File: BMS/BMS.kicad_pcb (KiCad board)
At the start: 2 copper layers, 15 x 15 mm, 17 parts, among them J1 Conn_01x02_Pin, J2 Conn_01x02_Pin, J3 Conn_01x02_Pin, Q1 A03401A, U1 MCP73831-2-OT, U2 XC6206PxxxMR

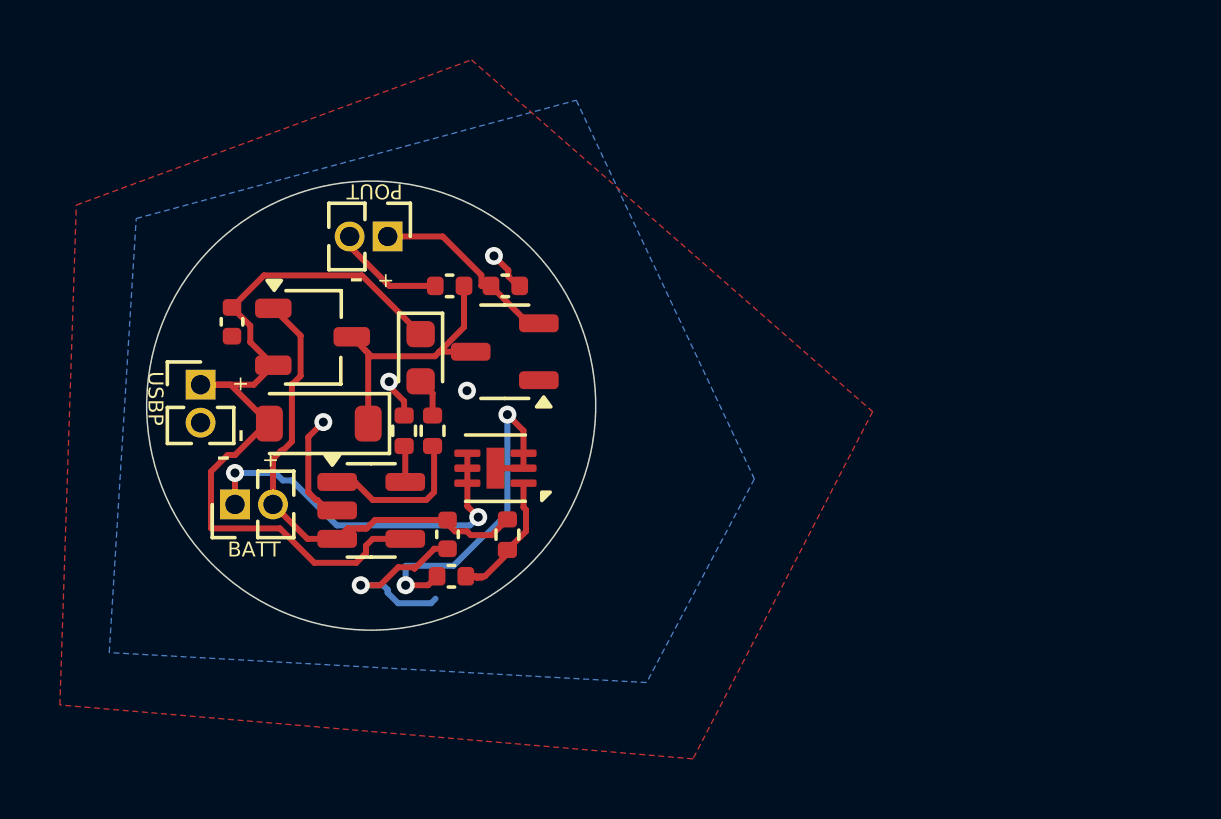
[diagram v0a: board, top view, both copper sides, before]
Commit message: BMS Rev 2
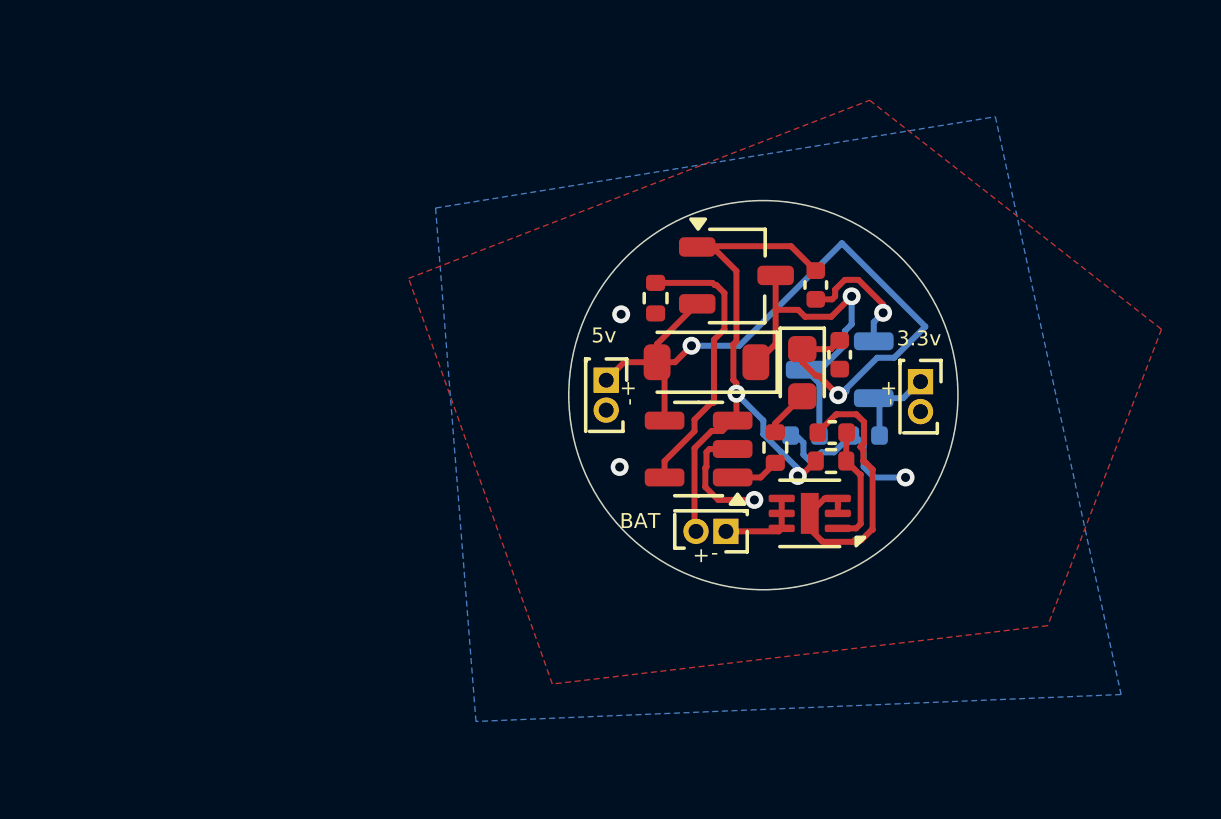
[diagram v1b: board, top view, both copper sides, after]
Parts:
- C2, C3, U2: moved to B.Cu
- J1, J2, J3: footprint Connector_PinHeader_1.27mm:PinHeader_1x02_P1.27mm_Vertical -> Connector_PinHeader_1.00mm:PinHeader_2x01_P1.00mm_Vertical
- moved C1 20.3 mm to (40.5, 17.9)
- moved J3 18.4 mm to (43.2, 18.9)
- moved J2 16.4 mm to (36.8, 23.9), turned to 180 degrees
- moved C4 14.9 mm to (39.8, 15.6)
- moved Q1 14.3 mm to (37.1, 15.3)
- moved C5 13.6 mm to (40.3, 20.6)
- moved J1 13.6 mm to (32.8, 18.8), turned to -90 degrees
- moved D1 13.1 mm to (36.1, 18.2)
- moved C3 13.0 mm to (41.4, 20.6), turned to 180 degrees
- moved C2 12.9 mm to (39.4, 20.6)
- moved D2 12.8 mm to (39.3, 18.6)
- moved R2 11.5 mm to (38.4, 21.1)
- moved U2 11.2 mm to (40.5, 18.4)
- moved U1 11.1 mm to (35.8, 21.1), turned to 180 degrees
- moved R3 11.1 mm to (40.3, 21.5), turned to 0 degrees
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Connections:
- net Net-(D1-K) renamed Vdrive
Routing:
- net Net-(J2-Pin_1): track 12.4 -> 2.90 mm, vias 2 -> 0
- net Net-(U1-PROG): track 1.22 -> 9.48 mm
- net Net-(U1-STAT): track 5.16 -> 1.63 mm
- net +3V3: track 6.46 -> 3.12 mm
- net VBAT: track 16.9 -> 19.9 mm, vias 0 -> 2
- net Vdrive: track 9.34 -> 11.9 mm, vias 0 -> 1
- net GND: track 16.6 -> 14.2 mm
- net VBUS: track 27.6 -> 25.7 mm, vias 0 -> 2
- net Net-(U3-EPAD): track 12.2 -> 10.4 mm, vias 2 -> 0
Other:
- board size 15 x 15 mm -> 13 x 13 mm
- board text added: "3.3v"
- board text added: "5v"
- board text added: "BAT"
- board text added: "MaxV: 5v"
- board text added: "Nixie Pendant BMS"
- board text added: "OutV: 3.3v"
- board text added: "Rev 2"
- board text removed: "BATT"
- board text removed: "POUT"
- board text removed: "USBP"

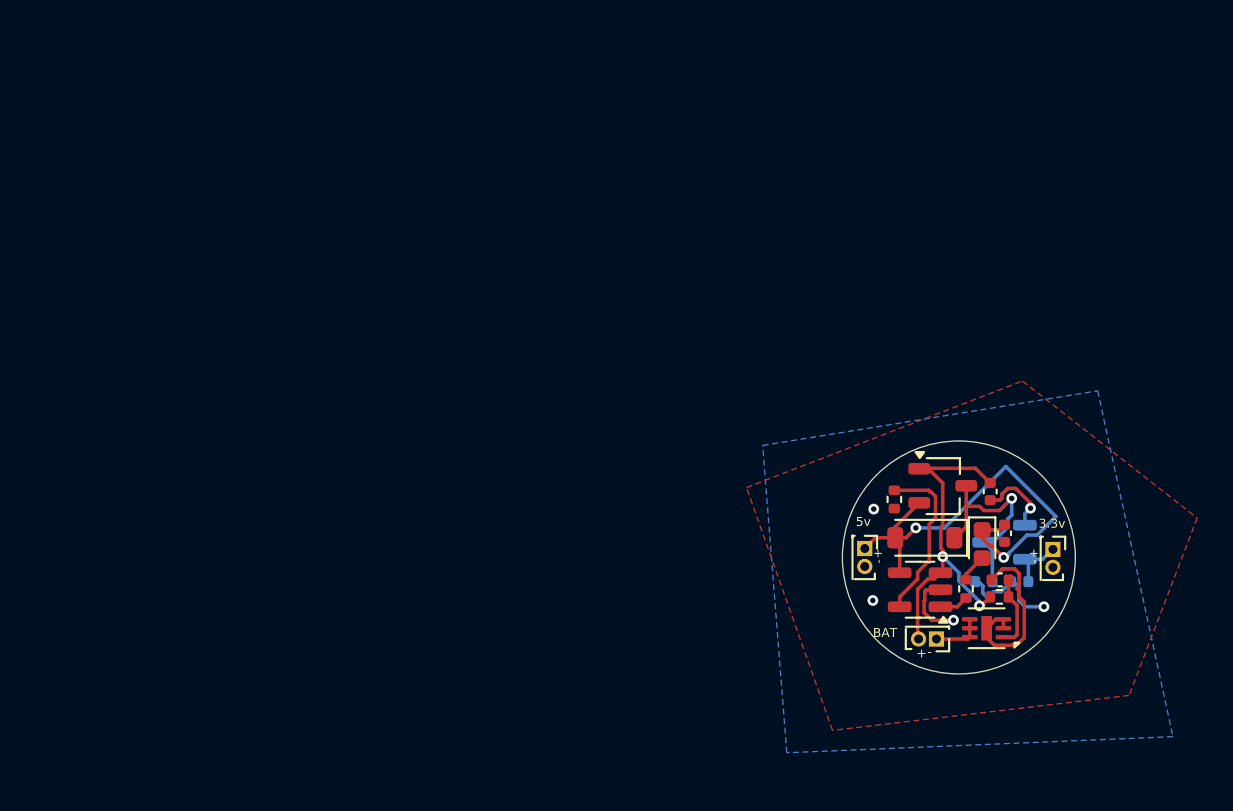
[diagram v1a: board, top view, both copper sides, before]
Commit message: Some BMS changes?, Socket PCB
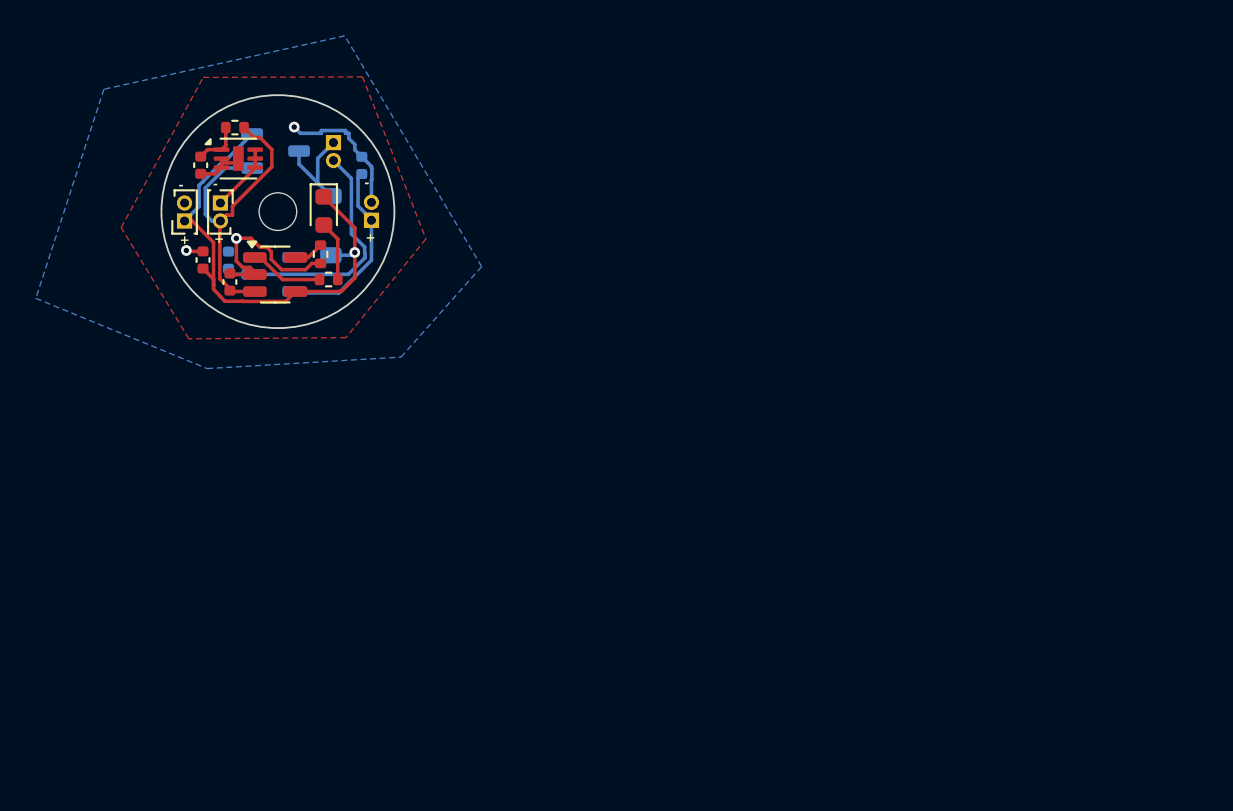
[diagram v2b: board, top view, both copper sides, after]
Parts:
- added H1: MountingHole, PendantLib:MountingHole_1.5mm, F.Cu at (0.00, 0.00)
- added SW1: SW_DPST_x2, Connector_PinHeader_1.00mm:PinHeader_2x01_P1.00mm_Vertical, B.Cu at (3.10, -3.85)
- D1, J3, Q1: moved to B.Cu
- moved C5 50.3 mm to (-4.31, -2.59), turned to -90 degrees
- moved R3 50.1 mm to (-2.40, -4.69), turned to 180 degrees
- moved U3 49.3 mm to (-2.21, -2.96), turned to 0 degrees
- moved C1 47.3 mm to (-4.18, 2.70), turned to 90 degrees
- moved J2 46.8 mm to (-3.21, -0.48), turned to -90 degrees
- moved C2 45.8 mm to (-2.76, 2.71), turned to 90 degrees
- moved C4 44.0 mm to (-2.68, 3.93), turned to 90 degrees
- moved C3 43.5 mm to (4.68, -2.58), turned to 90 degrees
- moved U2 43.4 mm to (-0.23, 3.50)
- moved J3 42.2 mm to (5.22, 0.48), turned to 90 degrees
- moved J1 42.1 mm to (-5.21, 0.52), turned to 90 degrees
- moved Q1 41.7 mm to (-0.13, -3.38)
- moved D2 41.2 mm to (2.56, -0.04)
- moved U1 40.1 mm to (-0.15, 3.51), turned to 0 degrees
- moved R2 39.5 mm to (2.83, 3.79), turned to 0 degrees
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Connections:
- D1 pad 1: Vdrive -> Net-(D1-K)
- Q1 pad 3: Vdrive -> Net-(D1-K)
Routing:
- net Net-(U1-PROG): track 9.48 -> 1.68 mm
- net Net-(U3-EPAD): track 10.4 -> 2.85 mm
- net +3V3: track 3.12 -> 10.5 mm
- net Net-(D1-K): track 0.00 -> 6.01 mm
- net GND: track 14.2 -> 18.8 mm, vias 5 -> 3
- net Net-(U1-STAT): track 1.63 -> 4.11 mm
- net Vdrive: track 11.9 -> 14.3 mm, vias 1 -> 0
- net VBUS: track 25.7 -> 27.8 mm, vias 2 -> 1
- net Net-(D2-A): track 1.58 -> 3.36 mm
- net Net-(U3-VDD): track 4.10 -> 2.65 mm
- net VBAT: track 19.9 -> 18.7 mm, vias 2 -> 0
- net Net-(J2-Pin_1): track 2.90 -> 3.78 mm
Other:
- board text removed: "3.3v"
- board text removed: "5v"
- board text removed: "BAT"
- board text removed: "MaxV: 5v"
- board text removed: "Nixie Pendant BMS"
- board text removed: "OutV: 3.3v"
- board text removed: "Rev 2"
